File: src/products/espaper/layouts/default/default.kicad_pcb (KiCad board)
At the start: 2 copper layers, 50 x 25 mm, 43 parts

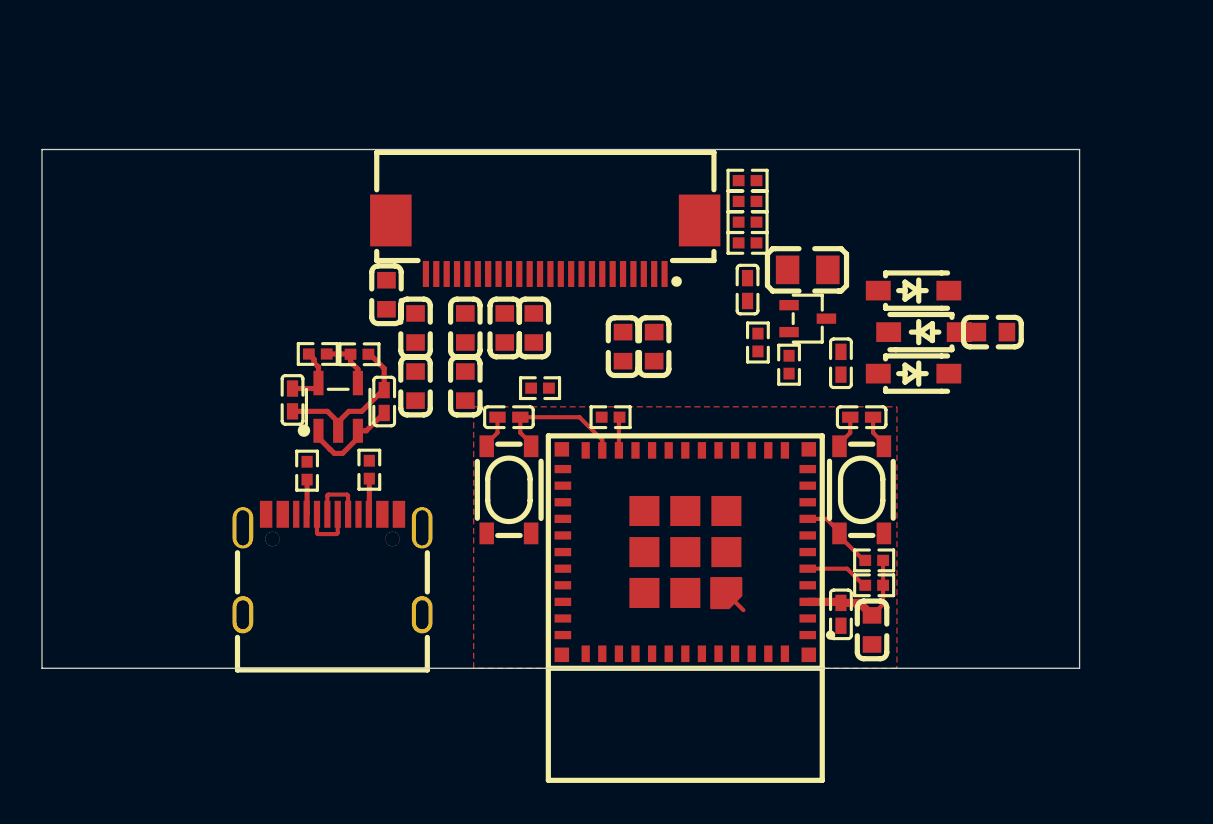
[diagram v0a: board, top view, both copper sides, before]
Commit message: almost done, need to finish a few traces
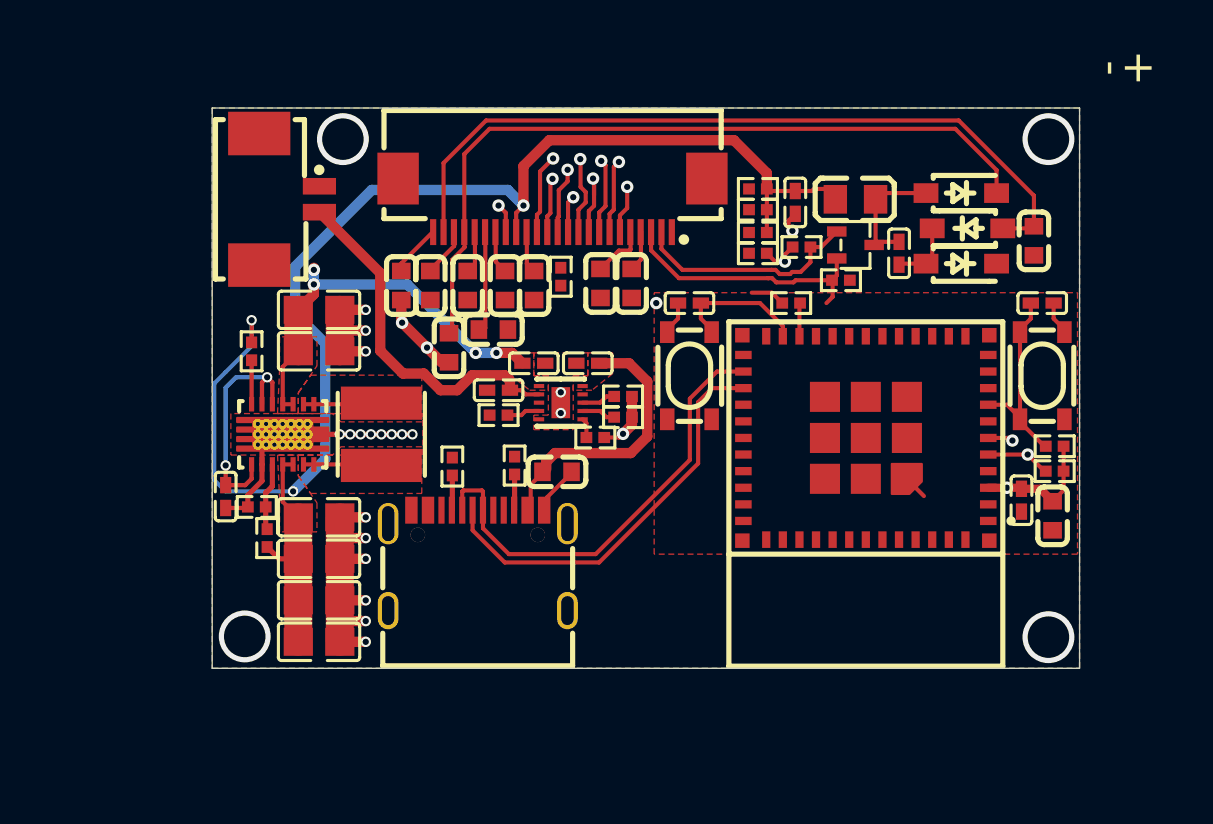
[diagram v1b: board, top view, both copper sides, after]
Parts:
- added B1: , EEMB_BATTERY_LP402535:EEMB_BATTERY_LP402535, B.Cu at (148.9, 101.3)
- added C19: 4.7µF ±10% 16V X5R, Samsung_Electro_Mechanics_CL10A475KO8NNNC:C0603, F.Cu at (144.8, 105.5)
- added C20: 22µF ±20% 6.3V X5R, Samsung_Electro_Mechanics_CL21A226MQQNNNE:C0805, F.Cu at (133.3, 113.7)
- added C21: 22µF ±20% 6.3V X5R, Samsung_Electro_Mechanics_CL21A226MQQNNNE:C0805, F.Cu at (133.3, 111.7)
- added C22: 22µF ±20% 6.3V X5R, Samsung_Electro_Mechanics_CL21A226MQQNNNE:C0805, F.Cu at (133.3, 109.7)
- added C23: 22µF ±20% 6.3V X5R, Samsung_Electro_Mechanics_CL21A226MQQNNNE:C0805, F.Cu at (133.3, 107.7)
- added C24: 100nF ±10% 16V X7R, Samsung_Electro_Mechanics_CL05B104KO5NNNC:C0402, F.Cu at (128.8, 106.7)
- added C25: 1µF ±10% 25V X5R, Samsung_Electro_Mechanics_CL05A105KA5NQNC:C0402, F.Cu at (142.0, 101.6)
- added C26: 10µF ±20% 6.3V X5R, Murata_Electronics_GRM155R60J106ME44D:C0402, F.Cu at (143.7, 100.3)
- added C27: 1µF ±10% 25V X5R, Samsung_Electro_Mechanics_CL05A105KA5NQNC:C0402, F.Cu at (146.3, 100.3)
- added L1: 1µH ±20% 4.7A 18mΩ, cjiang_FNR4030S1R0MT:IND-SMD_L4.0-W4.0_FNR40XXS, F.Cu at (136.3, 103.7)
- added R15: 2kΩ ±1% 62.5mW, UNI_ROYAL_0402WGF2001TCE:R0402, F.Cu at (148.0, 101.9)
- added R16: 10kΩ ±1% 62.5mW, UNI_ROYAL_0402WGF1002TCE:R0402, F.Cu at (142.0, 102.8)
- added R17: 18kΩ ±1% 62.5mW, UNI_ROYAL_0402WGF1802TCE:R0402, F.Cu at (148.0, 102.9)
- added R18: 10kΩ ±1% 62.5mW, UNI_ROYAL_0402WGF1002TCE:R0402, F.Cu at (145.0, 96.1)
- added R19: 10kΩ ±1% 62.5mW, UNI_ROYAL_0402WGF1002TCE:R0402, F.Cu at (146.7, 103.9)
- added U3: , Texas_Instruments_TPS63020DSJR:VSON-14_L4.0-W3.0-P0.50-BL-EP_TI_DSJ, F.Cu at (131.6, 103.7)
- added U4: , BQ25185DLHR_BQ25185DLHR:WSON-10_L2.2-W2.0-P0.40-BL-EP_TI_DLH0010A, F.Cu at (145.0, 102.2)
- C3, C4: value 1µF ±10% 25V X5R -> 10µF ±10% 25V X5R; footprint Samsung_Electro_Mechanics_CL05A105KA5NQNC:C0402 -> Samsung_Electro_Mechanics_CL21A106KAYNNNE:C0805
- R1: value 10kΩ ±1% 62.5mW -> 180kΩ ±1% 62.5mW; footprint UNI_ROYAL_0402WGF1002TCE:R0402 -> UNI_ROYAL_0402WGF1803TCE:R0402
- R2: value 18kΩ ±1% 62.5mW -> 1MΩ ±1% 62.5mW; footprint UNI_ROYAL_0402WGF1802TCE:R0402 -> UNI_ROYAL_0402WGF1004TCE:R0402
- R3: value 10kΩ ±1% 62.5mW -> 3.3Ω ±1% 62.5mW; footprint UNI_ROYAL_0402WGF1002TCE:R0402 -> UNI_ROYAL_0402WGF330KTCE:R0402
- R5: value 10kΩ ±1% 62.5mW -> 1MΩ ±1% 62.5mW; footprint UNI_ROYAL_0402WGF1002TCE:R0402 -> UNI_ROYAL_0402WGF1004TCE:R0402
- U1: footprint STMicroelectronics_LDK220M_R:SOT-23-5_L3.0-W1.7-P0.95-LS2.8-BL -> MOLEX_532610271:CONN-SMD_532610271
- moved R5 25.3 mm to (130.1, 99.7), turned to 90 degrees
- moved R12 13.6 mm to (154.5, 92.9)
- moved R7 10.3 mm to (168.8, 105.5)
- moved R9 10.3 mm to (168.8, 104.3)
- moved C14 10.3 mm to (151.2, 97.4)
- moved C15 10.3 mm to (168.2, 97.4)
- moved C16 10.3 mm to (168.7, 107.7)
- moved C17 10.3 mm to (167.2, 106.9)
- moved R8 10.3 mm to (156.1, 97.4)
- moved SW1 10.3 mm to (151.2, 100.9)
- moved SW2 10.3 mm to (168.2, 100.9)
- moved U2 10.3 mm to (159.7, 103.9)
- moved U1 10.3 mm to (131.9, 92.4), turned to 90 degrees
- moved R2 9.20 mm to (130.8, 108.7), turned to 90 degrees
- moved R1 8.87 mm to (130.3, 107.2), turned to 180 degrees
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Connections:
- C1 pad 1: -hv-0 -> -hv-1
- C10 pad 1: -line-7 -> cathode
- C11 pad 1: -line-8 -> -line-9
- C13 pad 1: -line-9 -> -line-10
- C16 pad 1: -hv-0 -> -hv-1
- C17 pad 1: -hv-0 -> -hv-1
- C3 pad 1: -hv-1 -> VIN
- C4 pad 1: -hv-0 -> VIN
- C5 pad 1: -line-3 -> -line-4
- C6 pad 1: cathode -> -line-5
- C7 pad 1: -line-4 -> -line-6
- C8 pad 1: -line-5 -> -line-7
- C9 pad 1: -line-6 -> -line-8
- FPC1 pad 10: -line-12 -> -line-11
- FPC1 pad 11: -line-2 -> -line-3
- FPC1 pad 12: output-0 -> -line-2
- FPC1 pad 13: -line-13 -> -line-12
- FPC1 pad 14: -line-14 -> -line-13
- FPC1 pad 16: -hv-0 -> -hv-1
- FPC1 pad 18: -line-4 -> -line-6
- FPC1 pad 19: -line-5 -> -line-7
- FPC1 pad 20: -line-6 -> -line-8
- FPC1 pad 21: -line-7 -> cathode
- FPC1 pad 22: -line-8 -> -line-9
- FPC1 pad 24: -line-9 -> -line-10
- FPC1 pad 4: -line-3 -> -line-4
- FPC1 pad 5: cathode -> -line-5
- L2 pad 1: -hv-0 -> -hv-1
- R1 pad 1: ADJ_NC -> FB
- R12 pad 1: -line-12 -> -line-11
- R12 pad 2: -hv-0 -> -hv-1
- R2 pad 1: -hv-0 -> -hv-1
- R2 pad 2: ADJ_NC -> FB
- R4 pad 2: -hv-0 -> -hv-1
- R5 pad 1: output-0 -> PG
- R5 pad 2: -hv-0 -> -hv-1
- R6 pad 1: -line-2 -> -line-3
- R6 pad 2: -hv-0 -> -hv-1
- R7 pad 1: -line-10 -> -line-1
- R7 pad 2: -hv-0 -> -hv-1
- R8 pad 1: -line-15 -> -line-14
- R8 pad 2: -hv-0 -> -hv-1
- R9 pad 1: -hv-0 -> -hv-1
- U1 pad 1: -hv-1 -> gnd
- U1 pad 2: gnd -> -hv-0
- U1 pad 3: -hv-1 -> gnd
- U1 pad 4: ADJ_NC -> gnd
- U2 pad 16: -line-13 -> -line-12
- U2 pad 18: -line-11 -> -line-3
- U2 pad 21: -line-14 -> -line-13
- U2 pad 22: -line-15 -> -line-14
- U2 pad 26: -line-17 -> -line-15
- U2 pad 27: -line-18 -> -line-16
- U2 pad 3: -hv-0 -> -hv-1
- U2 pad 5: -line-10 -> -line-1
- U2 pad 6: -line-16 -> -line-11
- USB1 pad A4: -hv-1 -> -hv-2
- USB1 pad A6: -line-18 -> -line-16
- USB1 pad A7: -line-17 -> -line-15
- USB1 pad A9: -hv-1 -> -hv-2
- USB1 pad B4: -hv-1 -> -hv-2
- USB1 pad B6: -line-18 -> -line-16
- USB1 pad B7: -line-17 -> -line-15
- USB1 pad B9: -hv-1 -> -hv-2
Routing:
- net -hv-1: track 4.83 -> 80.2 mm, vias 0 -> 4
- net gnd: track 12.6 -> 49.9 mm, vias 0 -> 25
- net -anode-1: track 0.00 -> 37.1 mm
- net cathode: track 0.00 -> 36.8 mm
- net -line-15: track 1.61 -> 22.2 mm
- net -line-16: track 0.00 -> 19.9 mm
- net VIN: track 0.00 -> 19.3 mm, vias 0 -> 4
- net -hv-2: track 0.00 -> 13.3 mm
- net source: track 0.00 -> 12.7 mm
- net EN: track 0.00 -> 11.8 mm, vias 0 -> 2
- net gate: track 0.00 -> 11.0 mm
- net -hv-0: track 9.34 -> 17.3 mm
- net -line-1: track 0.00 -> 6.65 mm, vias 0 -> 2
- net sw_node: track 0.00 -> 6.05 mm
- net -line-11: track 0.00 -> 5.55 mm, vias 0 -> 2
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- added copper zone on F.Cu, net (none)
- added copper zone on F.Cu, net -hv-1
- added copper zone on F.Cu, net -hv-2
- added copper zone on F.Cu, net L1
- added copper zone on F.Cu, net L2
- added copper zone on F.Cu, net VIN
- added copper zone on B.Cu, net gnd
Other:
- board size 50 x 25 mm -> 41.8 x 27 mm
- board text added: "+"
- board text added: "-"
